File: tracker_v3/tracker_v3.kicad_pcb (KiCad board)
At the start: 2 copper layers, 72 x 22.1 mm, 36 parts, among them J1 USB_C_Receptacle_PowerOnly_6P, J2 P70-7000045, J3 P70-7000045, Q1 DMG9926UDM-7, U1 XIAO-ESP32-DIP, U2 LIS3DH, U3 DW01A, U4 INA226AIDGSR, U5 TP4056-42-ESOP8

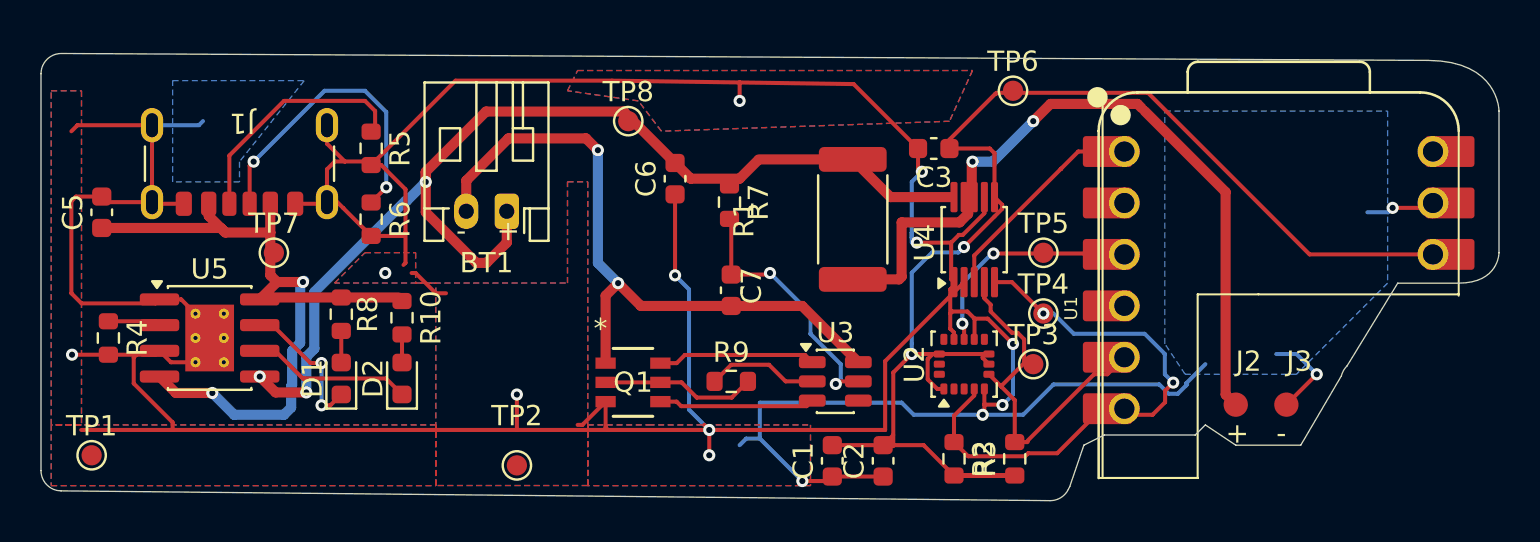
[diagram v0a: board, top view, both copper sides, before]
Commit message: v3.0 complete
the v3.0 has been added to cart for buying
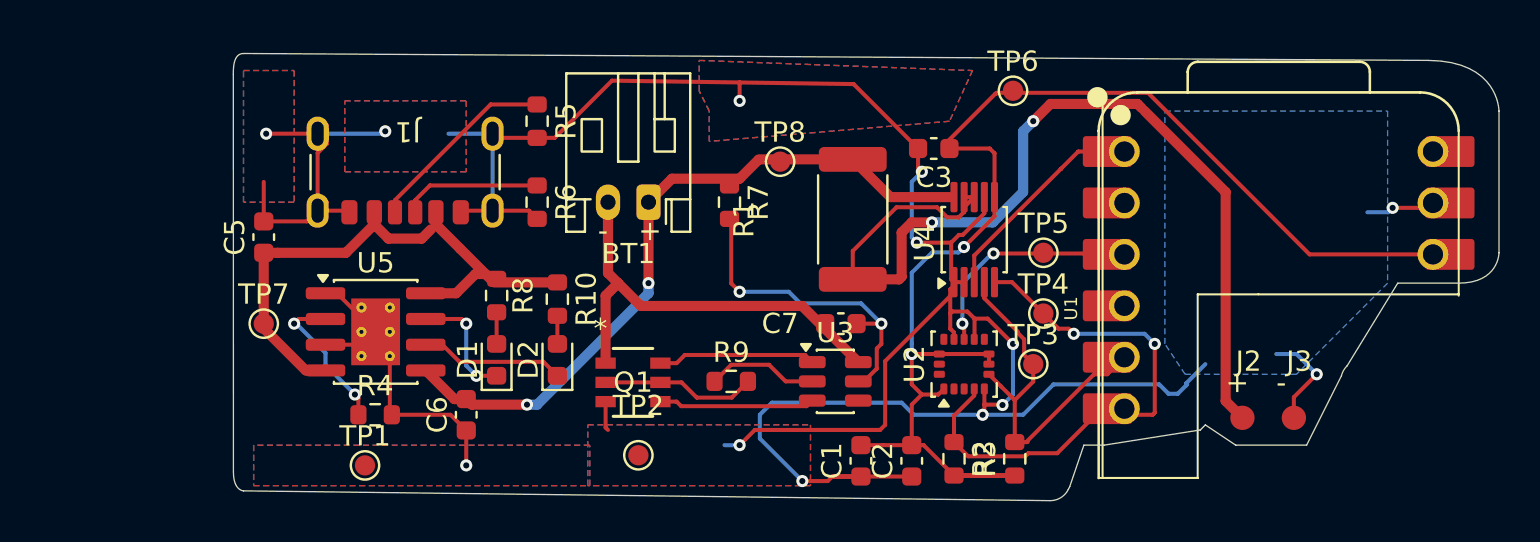
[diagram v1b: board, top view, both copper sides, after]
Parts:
- moved C6 15.6 mm to (143.0, 90.0)
- moved R4 13.7 mm to (138.5, 90.0), turned to 0 degrees
- moved TP1 13.5 mm to (138.0, 92.5)
- moved R5 8.31 mm to (146.5, 75.5)
- moved R6 8.24 mm to (146.5, 79.5)
- moved U5 8.20 mm to (138.5, 85.9)
- moved J1 8.19 mm to (140.0, 76.9)
- moved C5 8.09 mm to (133.0, 81.2)
- moved TP8 7.76 mm to (158.5, 77.5)
- moved D1 7.73 mm to (144.5, 87.3)
- moved D2 7.73 mm to (147.5, 87.3)
- moved R10 7.73 mm to (147.5, 84.3)
- moved R8 7.73 mm to (144.5, 84.1)
- moved BT1 7.01 mm to (152.0, 79.5)
- moved TP2 6.02 mm to (151.5, 92.0)
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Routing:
- net GND: track 223.5 -> 153.3 mm, vias 15 -> 13
- net /Charging_and_Battery/BAT+: track 54.8 -> 35.4 mm, vias 3 -> 2
- net /Charging_and_Battery/BAT-: track 33.8 -> 21.9 mm, vias 2 -> 0
- net /Shunt_Output: track 37.2 -> 48.4 mm
- net Net-(J1-CC1): track 15.4 -> 6.92 mm, vias 2 -> 0
- net USB_VBUS: track 37.6 -> 29.2 mm, vias 2 -> 0
- net Net-(U5-PROG): track 2.60 -> 7.52 mm, vias 0 -> 2
- net 3v3: track 68.6 -> 64.9 mm
- net Net-(U3-VCC): track 13.0 -> 16.0 mm
- net Net-(J1-CC2): track 12.0 -> 9.58 mm
- net (no net): track 2.11 -> 0.00 mm
- net Net-(D2-K): track 8.17 -> 7.14 mm
- net SCL: track 27.0 -> 26.3 mm
- net SDA: track 17.6 -> 18.2 mm
- net Net-(D1-K): track 6.48 -> 5.88 mm
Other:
- board size 72 x 22.1 mm -> 62.5 x 22.1 mm
